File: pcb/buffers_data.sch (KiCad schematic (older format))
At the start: 12 parts, among them U1 74LVCH162245A, U2 74LVCH162245A

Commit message: Some work done, sync
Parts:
- C1, C2, C3, C4, C5, C6, C7, C8: footprint Capacitor_SMD:C_0603_1608Metric_Pad1.05x0.95mm_HandSolder -> Capacitor_SMD:C_0402_1005Metric
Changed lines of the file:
@@
 F 0 "C1" V 3502 5200 50  0000 C CNN
 F 1 "0.1uF 35V" V 3411 5200 50  0000 C CNN
-F 2 "Capacitor_SMD:C_0603_1608Metric_Pad1.05x0.95mm_HandSolder" H 3288 5050 50  0001 C CNN
+F 2 "Capacitor_SMD:C_0402_1005Metric" H 3288 5050 50  0001 C CNN
 F 3 "~" H 3250 5200 50  0001 C CNN
 	1    3250 5200
@@
 F 0 "C3" V 3502 5600 50  0000 C CNN
 F 1 "0.1uF 35V" V 3411 5600 50  0000 C CNN
-F 2 "Capacitor_SMD:C_0603_1608Metric_Pad1.05x0.95mm_HandSolder" H 3288 5450 50  0001 C CNN
+F 2 "Capacitor_SMD:C_0402_1005Metric" H 3288 5450 50  0001 C CNN
 F 3 "~" H 3250 5600 50  0001 C CNN
 	1    3250 5600
@@
 F 0 "C5" V 3502 6000 50  0000 C CNN
 F 1 "0.1uF 35V" V 3411 6000 50  0000 C CNN
-F 2 "Capacitor_SMD:C_0603_1608Metric_Pad1.05x0.95mm_HandSolder" H 3288 5850 50  0001 C CNN
+F 2 "Capacitor_SMD:C_0402_1005Metric" H 3288 5850 50  0001 C CNN
 F 3 "~" H 3250 6000 50  0001 C CNN
 	1    3250 6000
@@
 F 0 "C7" V 3502 6400 50  0000 C CNN
 F 1 "0.1uF 35V" V 3411 6400 50  0000 C CNN
-F 2 "Capacitor_SMD:C_0603_1608Metric_Pad1.05x0.95mm_HandSolder" H 3288 6250 50  0001 C CNN
+F 2 "Capacitor_SMD:C_0402_1005Metric" H 3288 6250 50  0001 C CNN
 F 3 "~" H 3250 6400 50  0001 C CNN
 	1    3250 6400
@@
 F 0 "C2" V 8502 5200 50  0000 C CNN
 F 1 "0.1uF 35V" V 8411 5200 50  0000 C CNN
-F 2 "Capacitor_SMD:C_0603_1608Metric_Pad1.05x0.95mm_HandSolder" H 8288 5050 50  0001 C CNN
+F 2 "Capacitor_SMD:C_0402_1005Metric" H 8288 5050 50  0001 C CNN
 F 3 "~" H 8250 5200 50  0001 C CNN
 	1    8250 5200
@@
 F 0 "C4" V 8502 5600 50  0000 C CNN
 F 1 "0.1uF 35V" V 8411 5600 50  0000 C CNN
-F 2 "Capacitor_SMD:C_0603_1608Metric_Pad1.05x0.95mm_HandSolder" H 8288 5450 50  0001 C CNN
+F 2 "Capacitor_SMD:C_0402_1005Metric" H 8288 5450 50  0001 C CNN
 F 3 "~" H 8250 5600 50  0001 C CNN
 	1    8250 5600
@@
 F 0 "C6" V 8502 6000 50  0000 C CNN
 F 1 "0.1uF 35V" V 8411 6000 50  0000 C CNN
-F 2 "Capacitor_SMD:C_0603_1608Metric_Pad1.05x0.95mm_HandSolder" H 8288 5850 50  0001 C CNN
+F 2 "Capacitor_SMD:C_0402_1005Metric" H 8288 5850 50  0001 C CNN
 F 3 "~" H 8250 6000 50  0001 C CNN
 	1    8250 6000
@@
 F 0 "C8" V 8502 6400 50  0000 C CNN
 F 1 "0.1uF 35V" V 8411 6400 50  0000 C CNN
-F 2 "Capacitor_SMD:C_0603_1608Metric_Pad1.05x0.95mm_HandSolder" H 8288 6250 50  0001 C CNN
+F 2 "Capacitor_SMD:C_0402_1005Metric" H 8288 6250 50  0001 C CNN
 F 3 "~" H 8250 6400 50  0001 C CNN
 	1    8250 6400

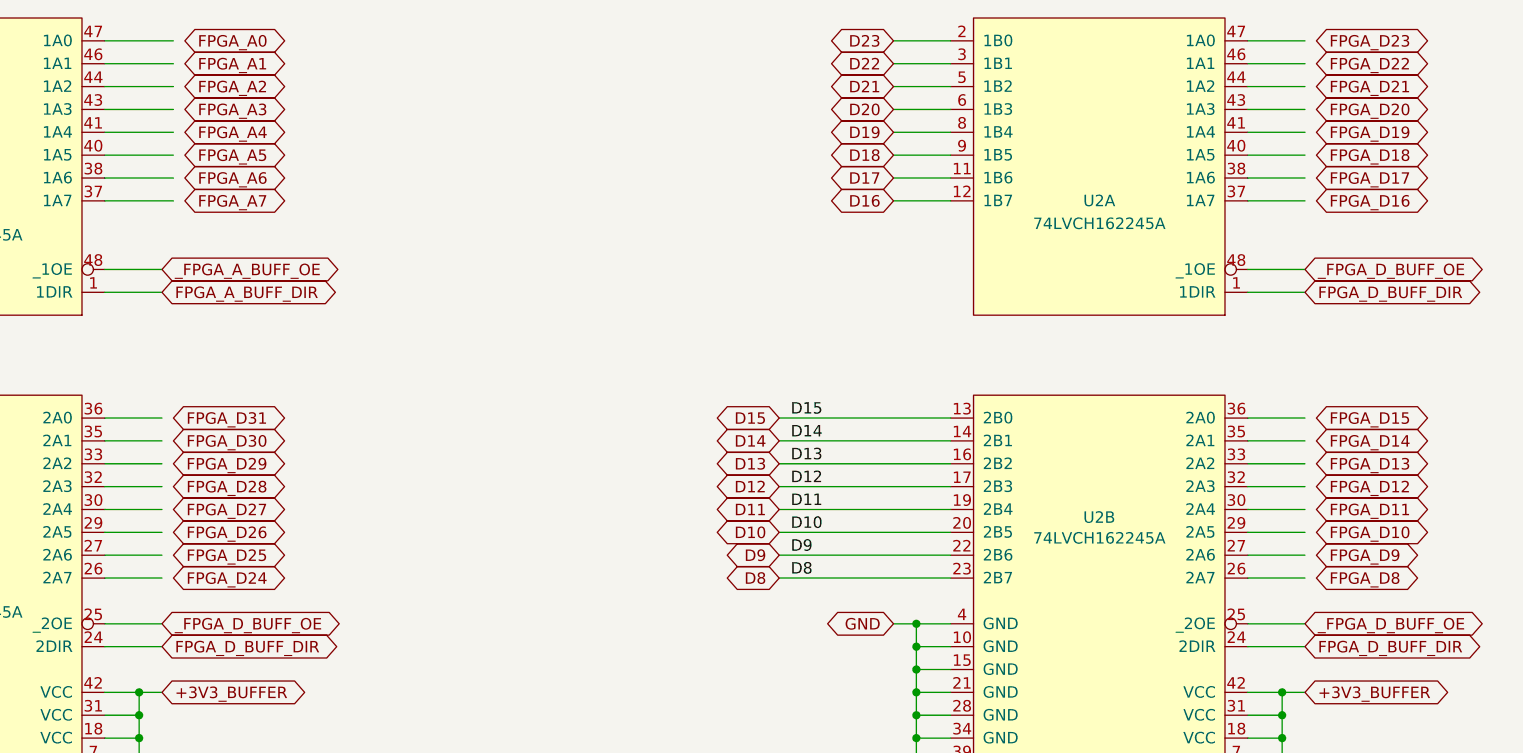
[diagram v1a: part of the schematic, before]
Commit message: some dirty routing
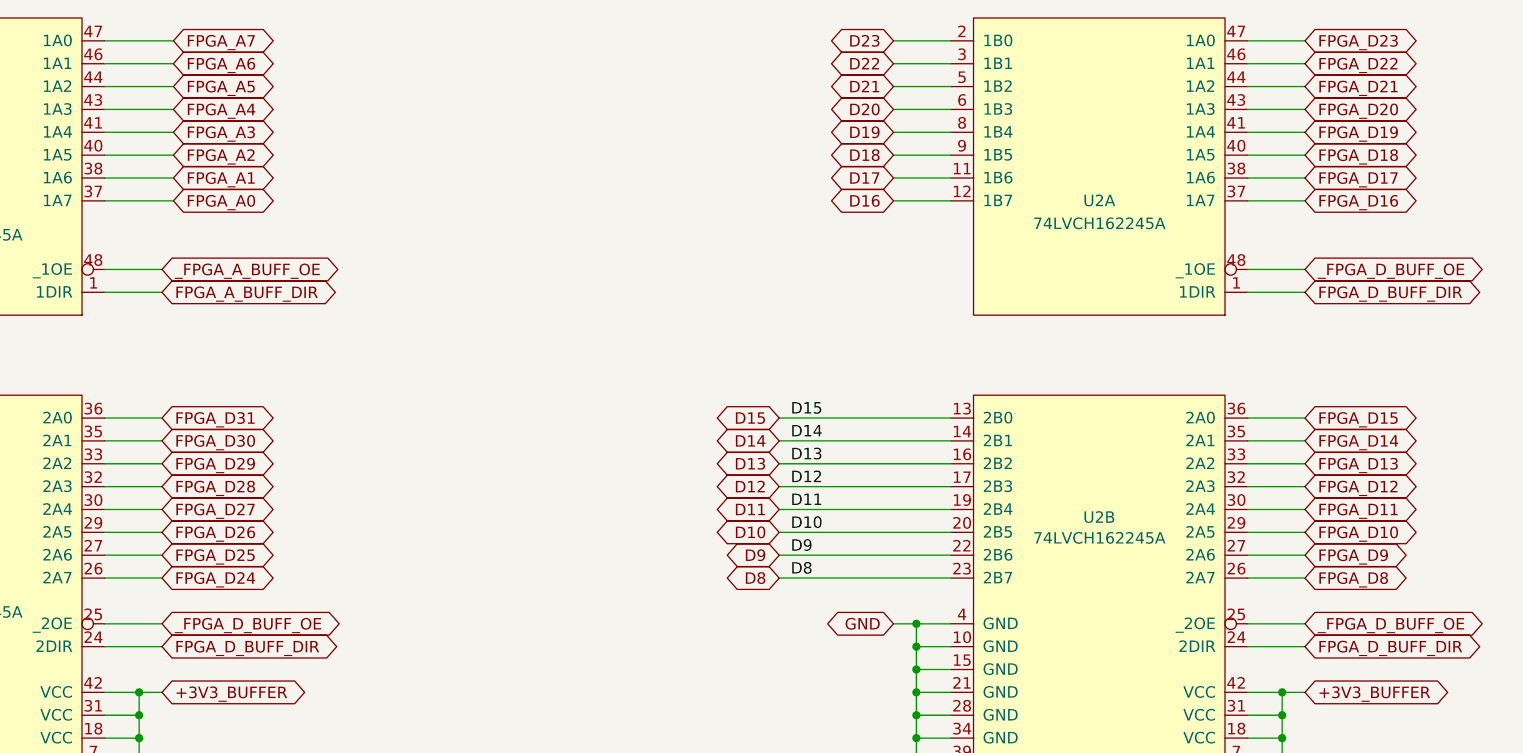
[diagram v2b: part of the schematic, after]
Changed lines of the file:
@@
 Text GLabel 9150 4200 2    50   BiDi ~ 0
 FPGA_D_BUFF_DIR
-Text GLabel 9200 1550 2    50   BiDi ~ 0
+Text GLabel 9150 1550 2    50   BiDi ~ 0
 FPGA_D23
-Text GLabel 9200 1650 2    50   BiDi ~ 0
+Text GLabel 9150 1650 2    50   BiDi ~ 0
 FPGA_D22
-Text GLabel 9200 1750 2    50   BiDi ~ 0
+Text GLabel 9150 1750 2    50   BiDi ~ 0
 FPGA_D21
-Text GLabel 9200 1850 2    50   BiDi ~ 0
+Text GLabel 9150 1850 2    50   BiDi ~ 0
 FPGA_D20
-Text GLabel 9200 1950 2    50   BiDi ~ 0
+Text GLabel 9150 1950 2    50   BiDi ~ 0
 FPGA_D19
-Text GLabel 9200 2050 2    50   BiDi ~ 0
+Text GLabel 9150 2050 2    50   BiDi ~ 0
 FPGA_D18
-Text GLabel 9200 2150 2    50   BiDi ~ 0
+Text GLabel 9150 2150 2    50   BiDi ~ 0
 FPGA_D17
-Text GLabel 9200 2250 2    50   BiDi ~ 0
+Text GLabel 9150 2250 2    50   BiDi ~ 0
 FPGA_D16
-Text GLabel 9200 3200 2    50   BiDi ~ 0
+Text GLabel 9150 3200 2    50   BiDi ~ 0
 FPGA_D15
-Text GLabel 9200 3300 2    50   BiDi ~ 0
+Text GLabel 9150 3300 2    50   BiDi ~ 0
 FPGA_D14
-Text GLabel 9200 3400 2    50   BiDi ~ 0
+Text GLabel 9150 3400 2    50   BiDi ~ 0
 FPGA_D13
-Text GLabel 9200 3500 2    50   BiDi ~ 0
+Text GLabel 9150 3500 2    50   BiDi ~ 0
 FPGA_D12
-Text GLabel 9200 3600 2    50   BiDi ~ 0
+Text GLabel 9150 3600 2    50   BiDi ~ 0
 FPGA_D11
-Text GLabel 9200 3700 2    50   BiDi ~ 0
+Text GLabel 9150 3700 2    50   BiDi ~ 0
 FPGA_D10
-Text GLabel 9200 3800 2    50   BiDi ~ 0
+Text GLabel 9150 3800 2    50   BiDi ~ 0
 FPGA_D9
-Text GLabel 9200 3900 2    50   BiDi ~ 0
+Text GLabel 9150 3900 2    50   BiDi ~ 0
 FPGA_D8
 Wire Wire Line
@@
 Wire Wire Line
 	4150 4100 3900 4100
-Text GLabel 4200 3900 2    50   BiDi ~ 0
+Text GLabel 4150 3900 2    50   BiDi ~ 0
 FPGA_D24
-Text GLabel 4200 3800 2    50   BiDi ~ 0
+Text GLabel 4150 3800 2    50   BiDi ~ 0
 FPGA_D25
-Text GLabel 4200 3700 2    50   BiDi ~ 0
+Text GLabel 4150 3700 2    50   BiDi ~ 0
 FPGA_D26
-Text GLabel 4200 3600 2    50   BiDi ~ 0
+Text GLabel 4150 3600 2    50   BiDi ~ 0
 FPGA_D27
-Text GLabel 4200 3500 2    50   BiDi ~ 0
+Text GLabel 4150 3500 2    50   BiDi ~ 0
 FPGA_D28
-Text GLabel 4200 3400 2    50   BiDi ~ 0
+Text GLabel 4150 3400 2    50   BiDi ~ 0
 FPGA_D29
-Text GLabel 4200 3300 2    50   BiDi ~ 0
+Text GLabel 4150 3300 2    50   BiDi ~ 0
 FPGA_D30
-Text GLabel 4200 3200 2    50   BiDi ~ 0
+Text GLabel 4150 3200 2    50   BiDi ~ 0
 FPGA_D31
 Text GLabel 4150 4200 2    50   BiDi ~ 0
@@
 Wire Wire Line
 	3900 3200 4150 3200
-Text GLabel 4250 1550 2    50   BiDi ~ 0
+Text GLabel 4200 2250 2    50   BiDi ~ 0
 FPGA_A0
-Text GLabel 4250 1650 2    50   BiDi ~ 0
+Text GLabel 4200 2150 2    50   BiDi ~ 0
 FPGA_A1
-Text GLabel 4250 1750 2    50   BiDi ~ 0
+Text GLabel 4200 2050 2    50   BiDi ~ 0
 FPGA_A2
-Text GLabel 4250 1850 2    50   BiDi ~ 0
+Text GLabel 4200 1950 2    50   BiDi ~ 0
 FPGA_A3
-Text GLabel 4250 1950 2    50   BiDi ~ 0
+Text GLabel 4200 1850 2    50   BiDi ~ 0
 FPGA_A4
-Text GLabel 4250 2050 2    50   BiDi ~ 0
+Text GLabel 4200 1750 2    50   BiDi ~ 0
 FPGA_A5
-Text GLabel 4250 2150 2    50   BiDi ~ 0
+Text GLabel 4200 1650 2    50   BiDi ~ 0
 FPGA_A6
-Text GLabel 4250 2250 2    50   BiDi ~ 0
+Text GLabel 4200 1550 2    50   BiDi ~ 0
 FPGA_A7
 Wire Wire Line
